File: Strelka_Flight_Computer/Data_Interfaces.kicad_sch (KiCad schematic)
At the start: 8 parts, among them J16 Conn_01x04, J6 USB_B_Micro, U8 MCP2551-I-SN, U8 USBLC6-2SC6

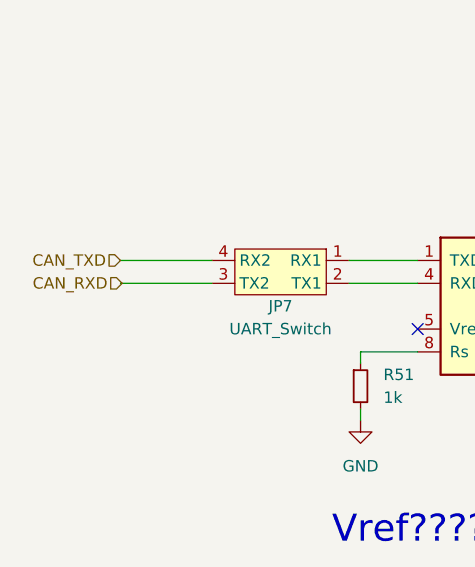
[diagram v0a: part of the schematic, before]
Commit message: Routing starting
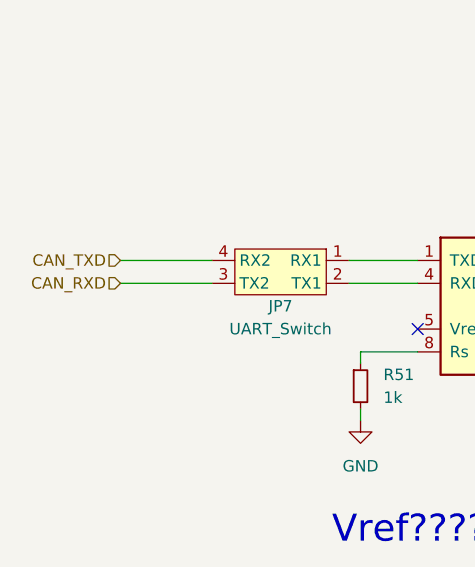
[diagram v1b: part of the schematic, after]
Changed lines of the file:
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@@
     (effects (font (size 1.27 1.27)) (justify right bottom))
   )
-  (hierarchical_label "CAN_RXD" (shape input) (at 81.4569 121.285 180) (fields_autoplaced)
+  (hierarchical_label "CAN_RXD" (shape input) (at 81.28 121.285 180) (fields_autoplaced)
     (effects (font (size 1.27 1.27)) (justify right))
   )
